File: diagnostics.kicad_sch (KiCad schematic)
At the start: 2 parts

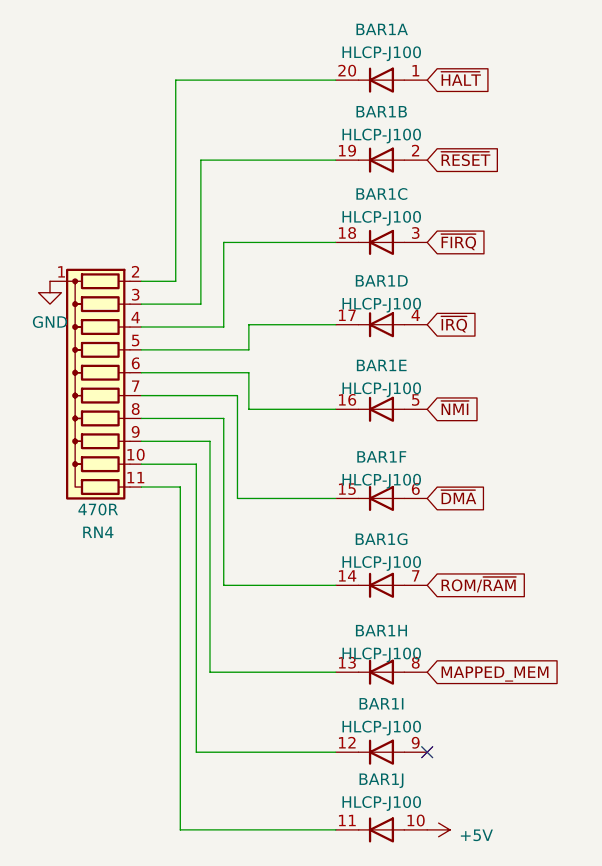
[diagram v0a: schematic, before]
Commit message: board refresh
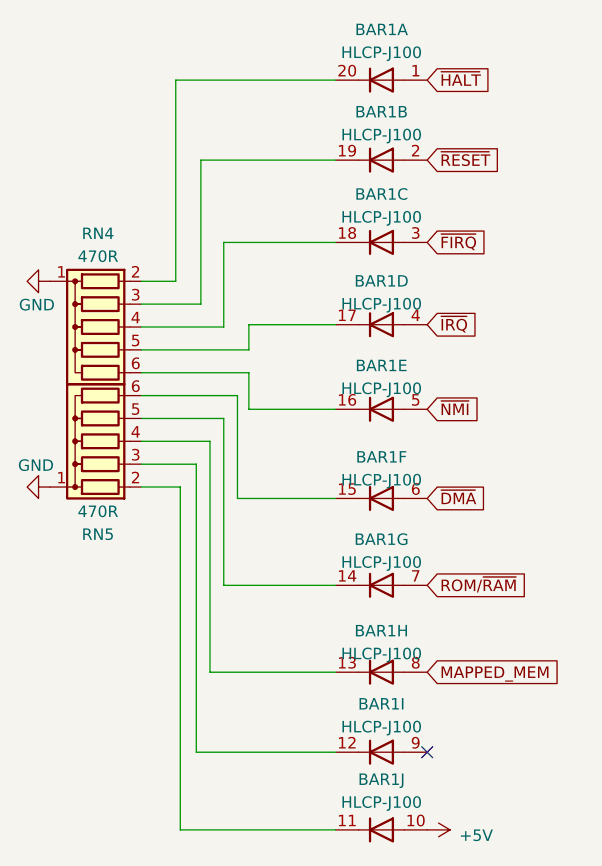
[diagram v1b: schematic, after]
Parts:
- removed RN4: 470R, Resistor_THT:R_Array_SIP11, symbol Device:R_Network10
- added RN4, RN5: 470R, Resistor_THT:R_Array_SIP6, symbol Device:R_Network05
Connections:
- net GND: now also RN4.1 (common), RN5.1 (common)
- net at BAR1.13 (K): now also RN5.4 (R3)
- net at BAR1.16 (K): now also RN4.6 (R5)
- net at BAR1.17 (K): now also RN4.5 (R4)
- net at BAR1.20 (K): now also RN4.2 (R1)
- net at BAR1.18 (K): now also RN4.4 (R3)
- net at BAR1.19 (K): now also RN4.3 (R2)
- net at BAR1.12 (K): now also RN5.3 (R2)
- net at BAR1.11 (K): now also RN5.2 (R1)
- net at BAR1.15 (K): now also RN5.6 (R5)
- net at BAR1.14 (K): now also RN5.5 (R4)
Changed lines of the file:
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@@
+    )
+  )
+  (symbol (lib_id "Device:R_Network05") (at 112.014 66.548 90) (mirror x) (unit 1)
+    (in_bom yes) (on_board yes) (dnp no) (fields_autoplaced)
+    (property "Reference" "RN4" (at 112.268 56.1848 90)
+      (effects (font (size 1.27 1.27)))
+    )
+    (property "Value" "470R" (at 112.268 58.7248 90)
+      (effects (font (size 1.27 1.27)))
+    )
+    (property "Footprint" "Resistor_THT:R_Array_SIP6" (at 112.014 76.073 90)
+      (effects (font (size 1.27 1.27)) hide)
+    )
+    (property "Datasheet" "http://www.vishay.com/docs/31509/csc.pdf" (at 112.014 66.548 0)
+      (effects (font (size 1.27 1.27)) hide)
+    )
+    (pin "1")
+    (pin "2")
+    (pin "3")
+    (pin "4")
+    (pin "5")
+    (pin "6")
+    (instances
+      (project "HD6309sbc"
+        (path "/b6976bcd-dc73-4942-aa19-f7adbf9104c7/d89ed66f-3f07-40a4-a82f-2642d873e0a8"
+          (reference "RN4") (unit 1)
+        )
+      )
+    )
+  )
+  (symbol (lib_id "power:GND") (at 106.934 84.328 270) (unit 1)
+    (in_bom yes) (on_board yes) (dnp no)
+    (property "Reference" "#PWR07" (at 100.584 84.328 0)
+      (effects (font (size 1.27 1.27)) hide)
+    )
+    (property "Value" "GND" (at 103.378 81.9404 90)
+      (effects (font (size 1.27 1.27)) (justify left))
+    )
+    (property "Footprint" "" (at 106.934 84.328 0)
+      (effects (font (size 1.27 1.27)) hide)
+    )
+    (property "Datasheet" "" (at 106.934 84.328 0)
+      (effects (font (size 1.27 1.27)) hide)
+    )
+    (pin "1")
+    (instances
+      (project "HD6309sbc"
+        (path "/b6976bcd-dc73-4942-aa19-f7adbf9104c7/d89ed66f-3f07-40a4-a82f-2642d873e0a8"
+          (reference "#PWR07") (unit 1)
+        )
+      )
     )
   )
@@
     )
   )
+  (symbol (lib_id "Device:R_Network05") (at 112.014 79.248 90) (unit 1)
+    (in_bom yes) (on_board yes) (dnp no)
+    (property "Reference" "RN5" (at 112.268 89.6112 90)
+      (effects (font (size 1.27 1.27)))
+    )
+    (property "Value" "470R" (at 112.268 87.0712 90)
+      (effects (font (size 1.27 1.27)))
+    )
+    (property "Footprint" "Resistor_THT:R_Array_SIP6" (at 112.014 69.723 90)
+      (effects (font (size 1.27 1.27)) hide)
+    )
+    (property "Datasheet" "http://www.vishay.com/docs/31509/csc.pdf" (at 112.014 79.248 0)
+      (effects (font (size 1.27 1.27)) hide)
+    )
+    (pin "1")
+    (pin "2")
+    (pin "3")
+    (pin "4")
+    (pin "5")
+    (pin "6")
+    (instances
+      (project "HD6309sbc"
+        (path "/b6976bcd-dc73-4942-aa19-f7adbf9104c7/d89ed66f-3f07-40a4-a82f-2642d873e0a8"
+          (reference "RN5") (unit 1)
+        )
+      )
+    )
+  )
   (symbol (lib_id "LED:HLCP-J100") (at 143.764 48.006 0) (mirror y) (unit 2)
     (in_bom yes) (on_board yes) (dnp no) (fields_autoplaced)
@@
     )
   )
-  (symbol (lib_id "Device:R_Network10") (at 112.014 74.168 90) (mirror x) (unit 1)
+  (symbol (lib_id "LED:HLCP-J100") (at 143.764 95.25 0) (mirror y) (unit 7)
+    (in_bom yes) (on_board yes) (dnp no) (fields_autoplaced)
+    (property "Reference" "BAR1" (at 143.764 90.17 0)
+      (effects (font (size 1.27 1.27)))
+    )
+    (property "Value" "HLCP-J100" (at 143.764 92.71 0)
+      (effects (font (size 1.27 1.27)))
+    )
+    (property "Footprint" "Display:HLCP-J100" (at 143.764 102.87 0)
+      (effects (font (size 1.27 1.27)) hide)
+    )
+    (property "Datasheet" "https://docs.broadcom.com/docs/AV02-1798EN" (at 143.764 95.25 0)
+      (effects (font (size 1.27 1.27)) hide)
+    )
+    (pin "1")
+    (pin "20")
+    (pin "19")
+    (pin "2")
+    (pin "18")
+    (pin "3")
+    (pin "17")
+    (pin "4")
+    (pin "16")
+    (pin "5")
+    (pin "15")
+    (pin "6")
+    (pin "14")
+    (pin "7")
+    (pin "13")
+    (pin "8")
+    (pin "12")
+    (pin "9")
+    (pin "10")
+    (pin "11")
+    (instances
+      (project "HD6309sbc"
+        (path "/b6976bcd-dc73-4942-aa19-f7adbf9104c7/d89ed66f-3f07-40a4-a82f-2642d873e0a8"
+          (reference "BAR1") (unit 7)
+        )
+      )
+    )
+  )
+  (symbol (lib_id "LED:HLCP-J100") (at 143.764 113.792 0) (mirror y) (unit 9)
+    (in_bom yes) (on_board yes) (dnp no) (fields_autoplaced)
+    (property "Reference" "BAR1" (at 143.764 108.458 0)
+      (effects (font (size 1.27 1.27)))
+    )
+    (property "Value" "HLCP-J100" (at 143.764 110.998 0)
+      (effects (font (size 1.27 1.27)))
+    )
+    (property "Footprint" "Display:HLCP-J100" (at 143.764 121.412 0)
+      (effects (font (size 1.27 1.27)) hide)
+    )
+    (property "Datasheet" "https://docs.broadcom.com/docs/AV02-1798EN" (at 143.764 113.792 0)
+      (effects (font (size 1.27 1.27)) hide)
+    )
+    (pin "1")
+    (pin "20")
+    (pin "19")
+    (pin "2")
+    (pin "18")
+    (pin "3")
+    (pin "17")
+    (pin "4")
+    (pin "16")
+    (pin "5")
+    (pin "15")
+    (pin "6")
+    (pin "14")
+    (pin "7")
+    (pin "13")
+    (pin "8")
+    (pin "12")
+    (pin "9")
+    (pin "10")
+    (pin "11")
+    (instances
+      (project "HD6309sbc"
+        (path "/b6976bcd-dc73-4942-aa19-f7adbf9104c7/d89ed66f-3f07-40a4-a82f-2642d873e0a8"
+          (reference "BAR1") (unit 9)
+        )
+      )
+    )
+  )
+  (symbol (lib_id "power:GND") (at 106.934 61.468 270) (unit 1)
     (in_bom yes) (on_board yes) (dnp no)
-    (property "Reference" "RN4" (at 112.268 89.408 90)
-      (effects (font (size 1.27 1.27)))
-    )
-    (property "Value" "470R" (at 112.268 86.868 90)
-      (effects (font (size 1.27 1.27)))
-    )
-    (property "Footprint" "Resistor_THT:R_Array_SIP11" (at 112.014 88.773 90)
-      (effects (font (size 1.27 1.27)) hide)
-    )
-    (property "Datasheet" "http://www.vishay.com/docs/31509/csc.pdf" (at 112.014 74.168 0)
-      (effects (font (size 1.27 1.27)) hide)
-    )
-    (pin "1")
-    (pin "10")
-    (pin "11")
-    (pin "2")
-    (pin "3")
-    (pin "4")
-    (pin "5")
-    (pin "6")
-    (pin "7")
-    (pin "8")
-    (pin "9")
-    (instances
-      (project "HD6309sbc"
-        (path "/b6976bcd-dc73-4942-aa19-f7adbf9104c7/d89ed66f-3f07-40a4-a82f-2642d873e0a8"
-          (reference "RN4") (unit 1)
-        )
-      )
-    )
-  )
-  (symbol (lib_id "LED:HLCP-J100") (at 143.764 95.25 0) (mirror y) (unit 7)
-    (in_bom yes) (on_board yes) (dnp no) (fields_autoplaced)
-    (property "Reference" "BAR1" (at 143.764 90.17 0)
-      (effects (font (size 1.27 1.27)))
-    )
-    (property "Value" "HLCP-J100" (at 143.764 92.71 0)
-      (effects (font (size 1.27 1.27)))
-    )
-    (property "Footprint" "Display:HLCP-J100" (at 143.764 102.87 0)
-      (effects (font (size 1.27 1.27)) hide)
-    )
-    (property "Datasheet" "https://docs.broadcom.com/docs/AV02-1798EN" (at 143.764 95.25 0)
-      (effects (font (size 1.27 1.27)) hide)
-    )
-    (pin "1")
-    (pin "20")
-    (pin "19")
-    (pin "2")
-    (pin "18")
-    (pin "3")
-    (pin "17")
-    (pin "4")
-    (pin "16")
-    (pin "5")
-    (pin "15")
-    (pin "6")
-    (pin "14")
-    (pin "7")
-    (pin "13")
-    (pin "8")
-    (pin "12")
-    (pin "9")
-    (pin "10")
-    (pin "11")
-    (instances
-      (project "HD6309sbc"
-        (path "/b6976bcd-dc73-4942-aa19-f7adbf9104c7/d89ed66f-3f07-40a4-a82f-2642d873e0a8"
-          (reference "BAR1") (unit 7)
-        )
-      )
-    )
-  )
-  (symbol (lib_id "LED:HLCP-J100") (at 143.764 113.792 0) (mirror y) (unit 9)
-    (in_bom yes) (on_board yes) (dnp no) (fields_autoplaced)
-    (property "Reference" "BAR1" (at 143.764 108.458 0)
-      (effects (font (size 1.27 1.27)))
-    )
-    (property "Value" "HLCP-J100" (at 143.764 110.998 0)
-      (effects (font (size 1.27 1.27)))
-    )
-    (property "Footprint" "Display:HLCP-J100" (at 143.764 121.412 0)
-      (effects (font (size 1.27 1.27)) hide)
-    )
-    (property "Datasheet" "https://docs.broadcom.com/docs/AV02-1798EN" (at 143.764 113.792 0)
-      (effects (font (size 1.27 1.27)) hide)
-    )
-    (pin "1")
-    (pin "20")
-    (pin "19")
-    (pin "2")
-    (pin "18")
-    (pin "3")
-    (pin "17")
-    (pin "4")
-    (pin "16")
-    (pin "5")
-    (pin "15")
-    (pin "6")
-    (pin "14")
-    (pin "7")
-    (pin "13")
-    (pin "8")
-    (pin "12")
-    (pin "9")
-    (pin "10")
-    (pin "11")
-    (instances
-      (project "HD6309sbc"
-        (path "/b6976bcd-dc73-4942-aa19-f7adbf9104c7/d89ed66f-3f07-40a4-a82f-2642d873e0a8"
-          (reference "BAR1") (unit 9)
-        )
-      )
-    )
-  )
-  (symbol (lib_id "power:GND") (at 106.934 61.468 0) (unit 1)
-    (in_bom yes) (on_board yes) (dnp no) (fields_autoplaced)
-    (property "Reference" "#PWR05" (at 106.934 67.818 0)
-      (effects (font (size 1.27 1.27)) hide)
-    )
-    (property "Value" "GND" (at 106.934 66.04 0)
-      (effects (font (size 1.27 1.27)))
+    (property "Reference" "#PWR05" (at 100.584 61.468 0)
+      (effects (font (size 1.27 1.27)) hide)
+    )
+    (property "Value" "GND" (at 103.4796 64.1096 90)
+      (effects (font (size 1.27 1.27)) (justify left))
     )
     (property "Footprint" "" (at 106.934 61.468 0)
